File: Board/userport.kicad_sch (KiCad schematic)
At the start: 24 parts, among them J4 Conn_01x02, P1 PETUSERPORT, U14 74LS06, U16 LSF0204Q, U17 LSF0204Q, U18 LSF0204Q, U19 LSF0204Q, U23 74LVC1G00, U26 CD4053B, U27 CD4053B, X7 M09-182, X8 M09-182

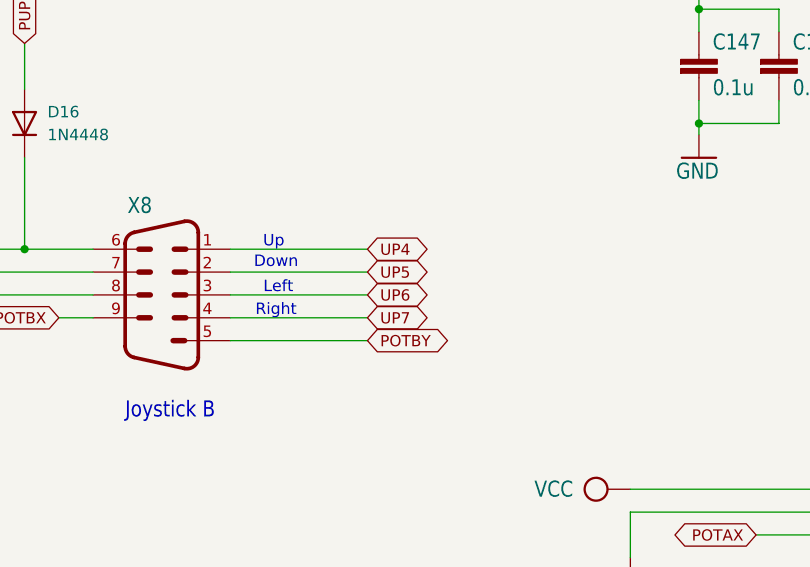
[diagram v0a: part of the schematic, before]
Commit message: more layout work
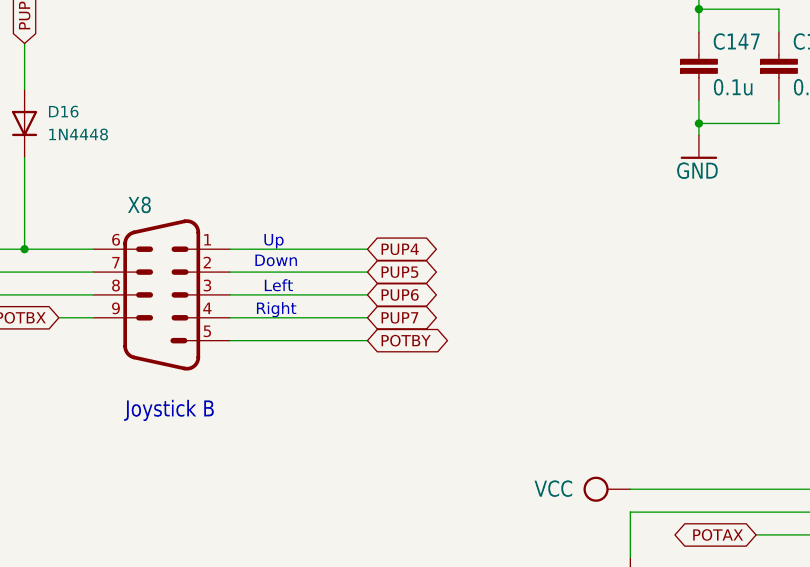
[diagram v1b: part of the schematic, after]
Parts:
- added unit 4 of U14
- X7, X8: LCSC (none) -> C189688
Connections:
- net PUP4: now also X8.1
- net PUP5: now also X8.2
- net PUP6: now also X8.3
- net PUP7: now also X8.4
- net UP4: no longer X8.1
- net UP5: no longer X8.2
- net UP6: no longer X8.3
- net UP7: no longer X8.4
- net at J4.2 (Pin_2): now also U14.9; no longer U14.9
- net at R10.2, U14.11: now also U14.8; no longer U14.8
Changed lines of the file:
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@@
 		)
 	)
-	(global_label "UP4"
+	(global_label "PUP4"
 		(shape bidirectional)
 		(at 223.52 67.31 0)
@@
 		)
 		(property "Intersheetrefs" "${INTERSHEET_REFS}"
-			(at 231.268 67.31 0)
+			(at 232.5126 67.31 0)
 			(hide yes)
 			(show_name no)
@@
 		)
 	)
-	(global_label "UP6"
+	(global_label "PUP6"
 		(shape bidirectional)
 		(at 223.52 72.39 0)
@@
 		)
 		(property "Intersheetrefs" "${INTERSHEET_REFS}"
-			(at 231.268 72.39 0)
+			(at 232.5126 72.39 0)
 			(hide yes)
 			(show_name no)
@@
 		)
 	)
-	(global_label "UP7"
+	(global_label "PUP7"
 		(shape bidirectional)
 		(at 223.52 74.93 0)
@@
 		)
 		(property "Intersheetrefs" "${INTERSHEET_REFS}"
-			(at 231.268 74.93 0)
+			(at 232.5126 74.93 0)
 			(hide yes)
 			(show_name no)
@@
 		)
 	)
-	(global_label "UP5"
+	(global_label "PUP5"
 		(shape bidirectional)
 		(at 223.52 69.85 0)
@@
 		)
 		(property "Intersheetrefs" "${INTERSHEET_REFS}"
-			(at 231.268 69.85 0)
+			(at 232.5126 69.85 0)
 			(hide yes)
 			(show_name no)
@@
 			)
 		)
+		(property "LCSC" "C189688"
+			(at 200.66 72.39 0)
+			(hide yes)
+			(show_name no)
+			(do_not_autoplace no)
+			(effects
+				(font
+					(size 1.27 1.27)
+				)
+			)
+		)
 		(pin "2"
 		)
@@
 			(at 283.21 96.52 0)
 			(hide yes)
+			(show_name no)
+			(do_not_autoplace no)
+			(effects
+				(font
+					(size 1.27 1.27)
+				)
+			)
+		)
+		(property "LCSC" "C189688"
+			(at 283.21 96.52 0)
+			(hide yes)
